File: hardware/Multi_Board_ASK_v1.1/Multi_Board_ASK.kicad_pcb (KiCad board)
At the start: 2 copper layers, 52.7 x 61.6 mm, 20 parts, among them J1 feather long, J2 feather short, J3 Nano 2, J4 Nano 1, J5 Pico 1, J6 Pico 2, P1 Power, P2 Analog, P3 Digital, P4 Digital, U1 Feather_Cu, U10 Feather_Silks, U11 KiCadLogo, U3 KiCadLogo, U4 Moon_Firma, U5 Feather_Silks, U6 KiCadLogo, U7 Feather_Cu, U8 KiCadLogo, U9 Moon_Firma

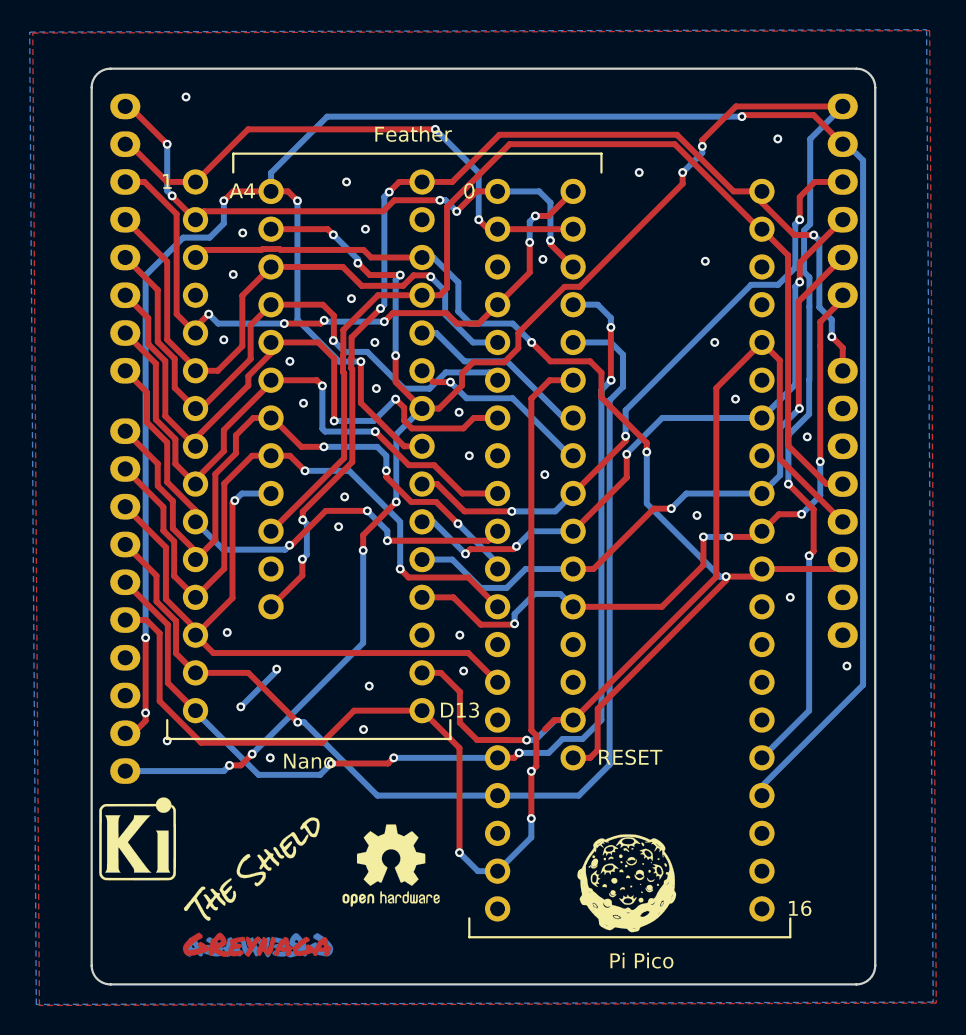
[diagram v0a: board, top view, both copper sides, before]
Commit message: Some changes
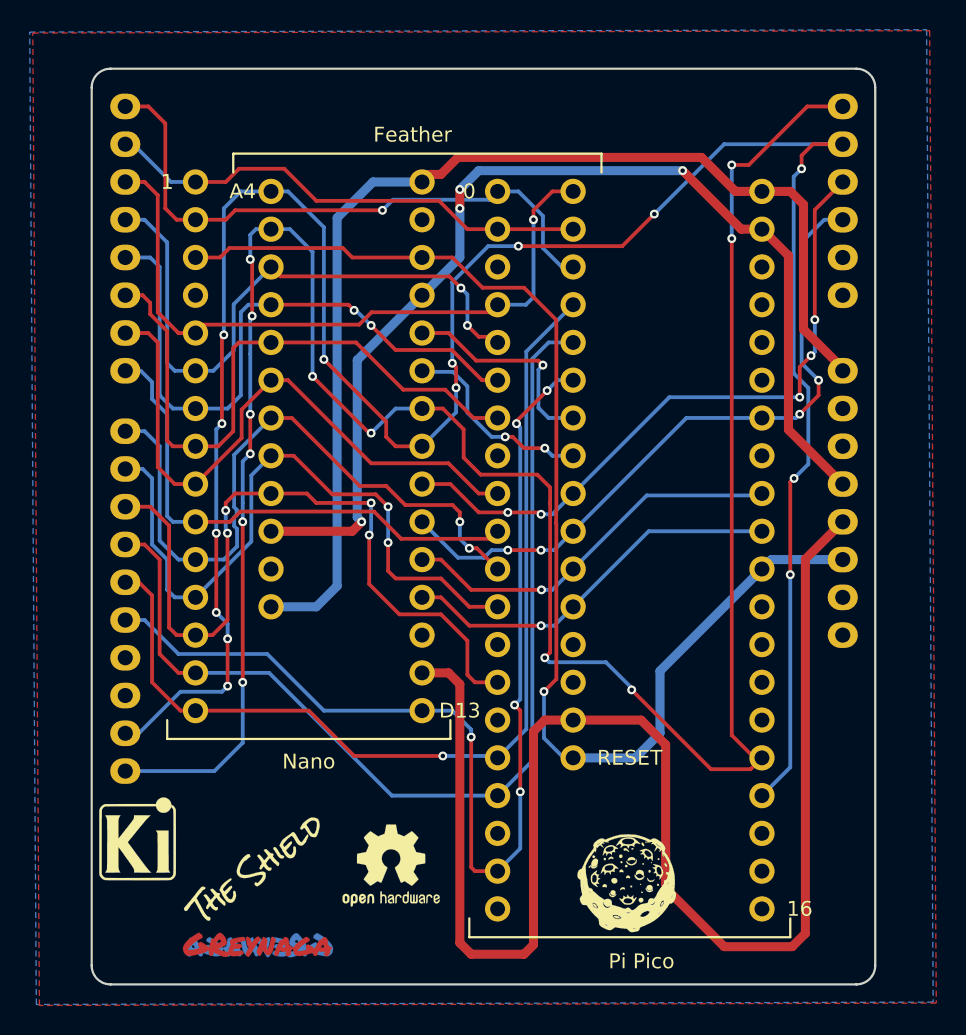
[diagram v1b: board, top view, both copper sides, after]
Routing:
- net +3V3: track 61.0 -> 99.8 mm, vias 1 -> 0
- net /A0: track 48.0 -> 26.3 mm, vias 5 -> 1
- net /A1: track 44.4 -> 26.4 mm, vias 2 -> 1
- net /SCL-A5: track 143.4 -> 157.9 mm
- net /~RESET: track 75.0 -> 83.6 mm, vias 3 -> 1
- net /D10(**): track 45.0 -> 51.3 mm, vias 1 -> 4
- net /D12-MISO: track 71.5 -> 65.9 mm, vias 5 -> 1
- net /D11-MOSI: track 74.4 -> 69.3 mm, vias 1 -> 0
- net /1(Tx): track 38.2 -> 33.2 mm, vias 2 -> 0
- net GND: track 3.54 -> 0.00 mm, vias 35 -> 0
- net /D13-SCK: track 77.0 -> 73.7 mm, vias 3 -> 5
- net /A3: track 42.0 -> 45.2 mm, vias 3 -> 5
- net /D8: track 43.4 -> 45.6 mm, vias 3 -> 2
- net /A7: track 12.5 -> 14.6 mm, vias 0 -> 1
- net /D4: track 40.7 -> 42.6 mm, vias 1 -> 2
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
